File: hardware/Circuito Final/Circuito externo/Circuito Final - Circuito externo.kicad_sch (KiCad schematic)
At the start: 74 parts, among them J1 Conn_02x19_Odd_Even, J2 Conn_02x19_Odd_Even, J3 Conn_01x02, J4 Conn_01x02, J5 Conn_01x03_Pin, Q1 FDMS6681Z, Q2 FDMS6681Z, Q3 MMBT2222A, SW1 SW_SPDT, SW2 SW_DIP_x04, SW3 SW_DIP_x04, SW4 SW_DIP_x01, SW5 SW_DIP_x01, SW6 SW_DIP_x01, U1 Opamp_Quad, U2 ICL7660, U3 INA180A1

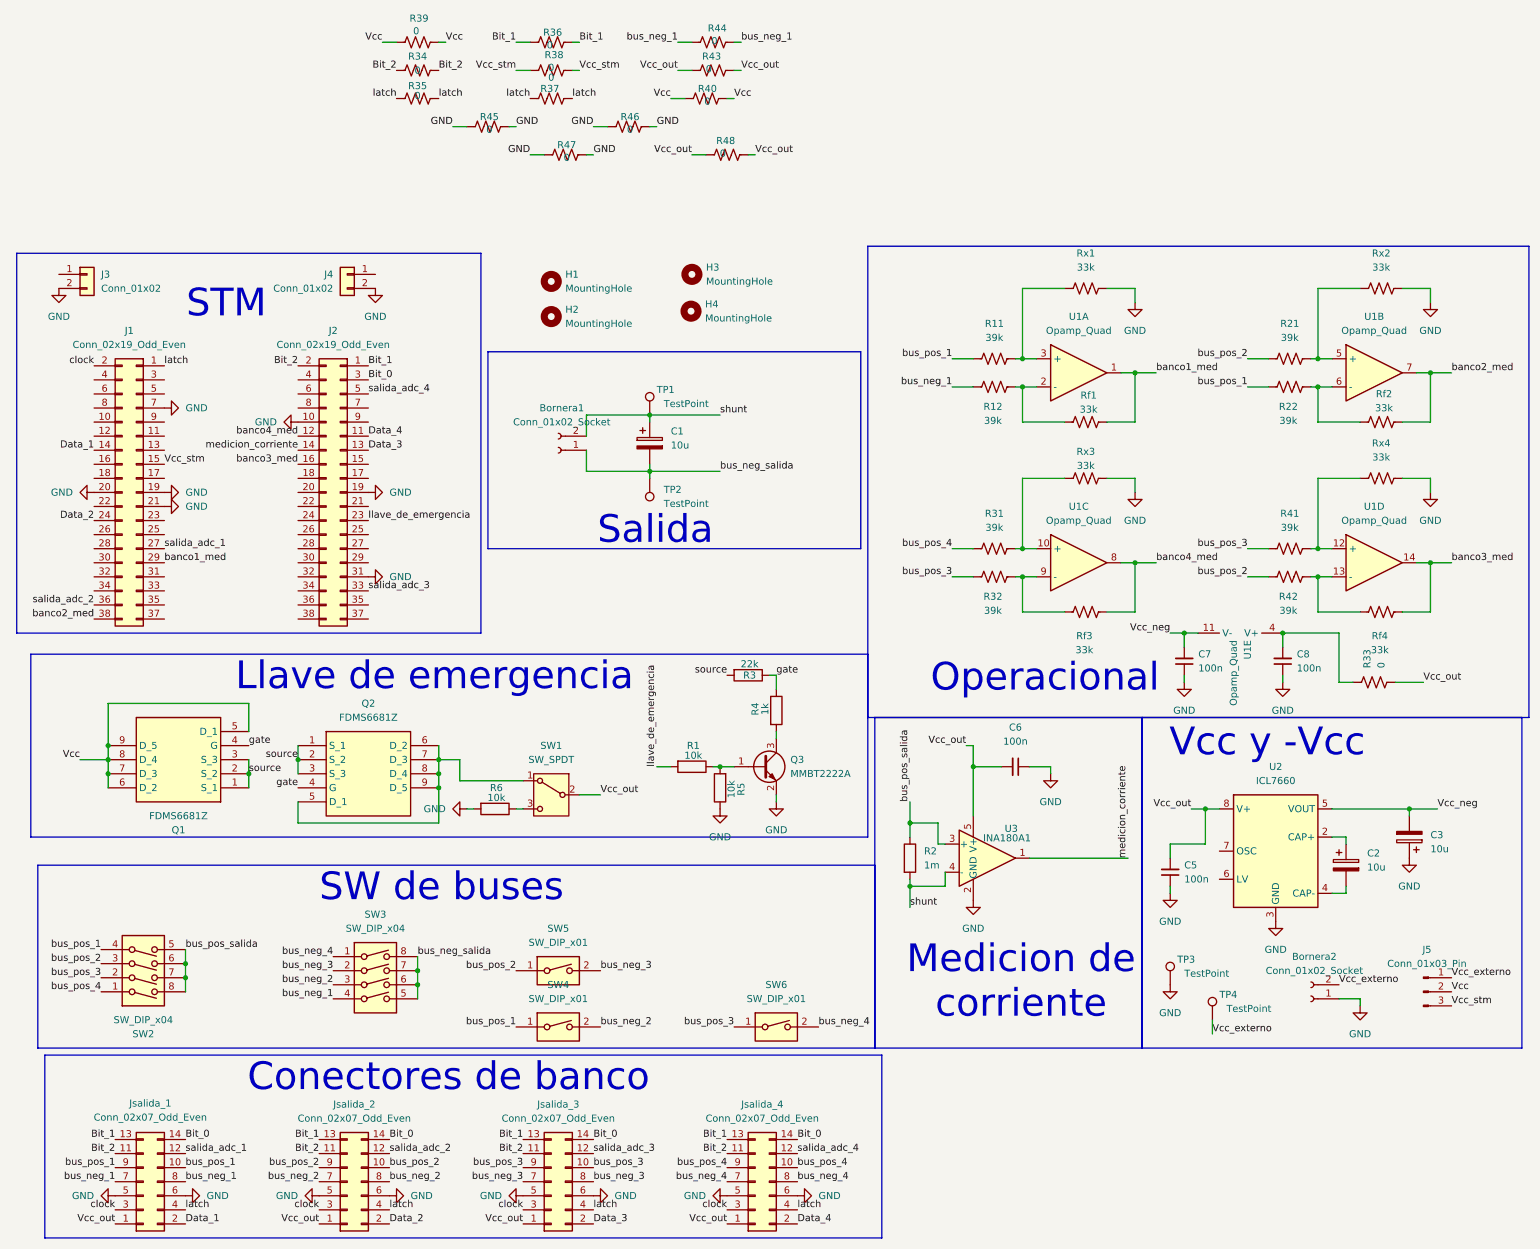
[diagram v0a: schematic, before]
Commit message: listo la placa central
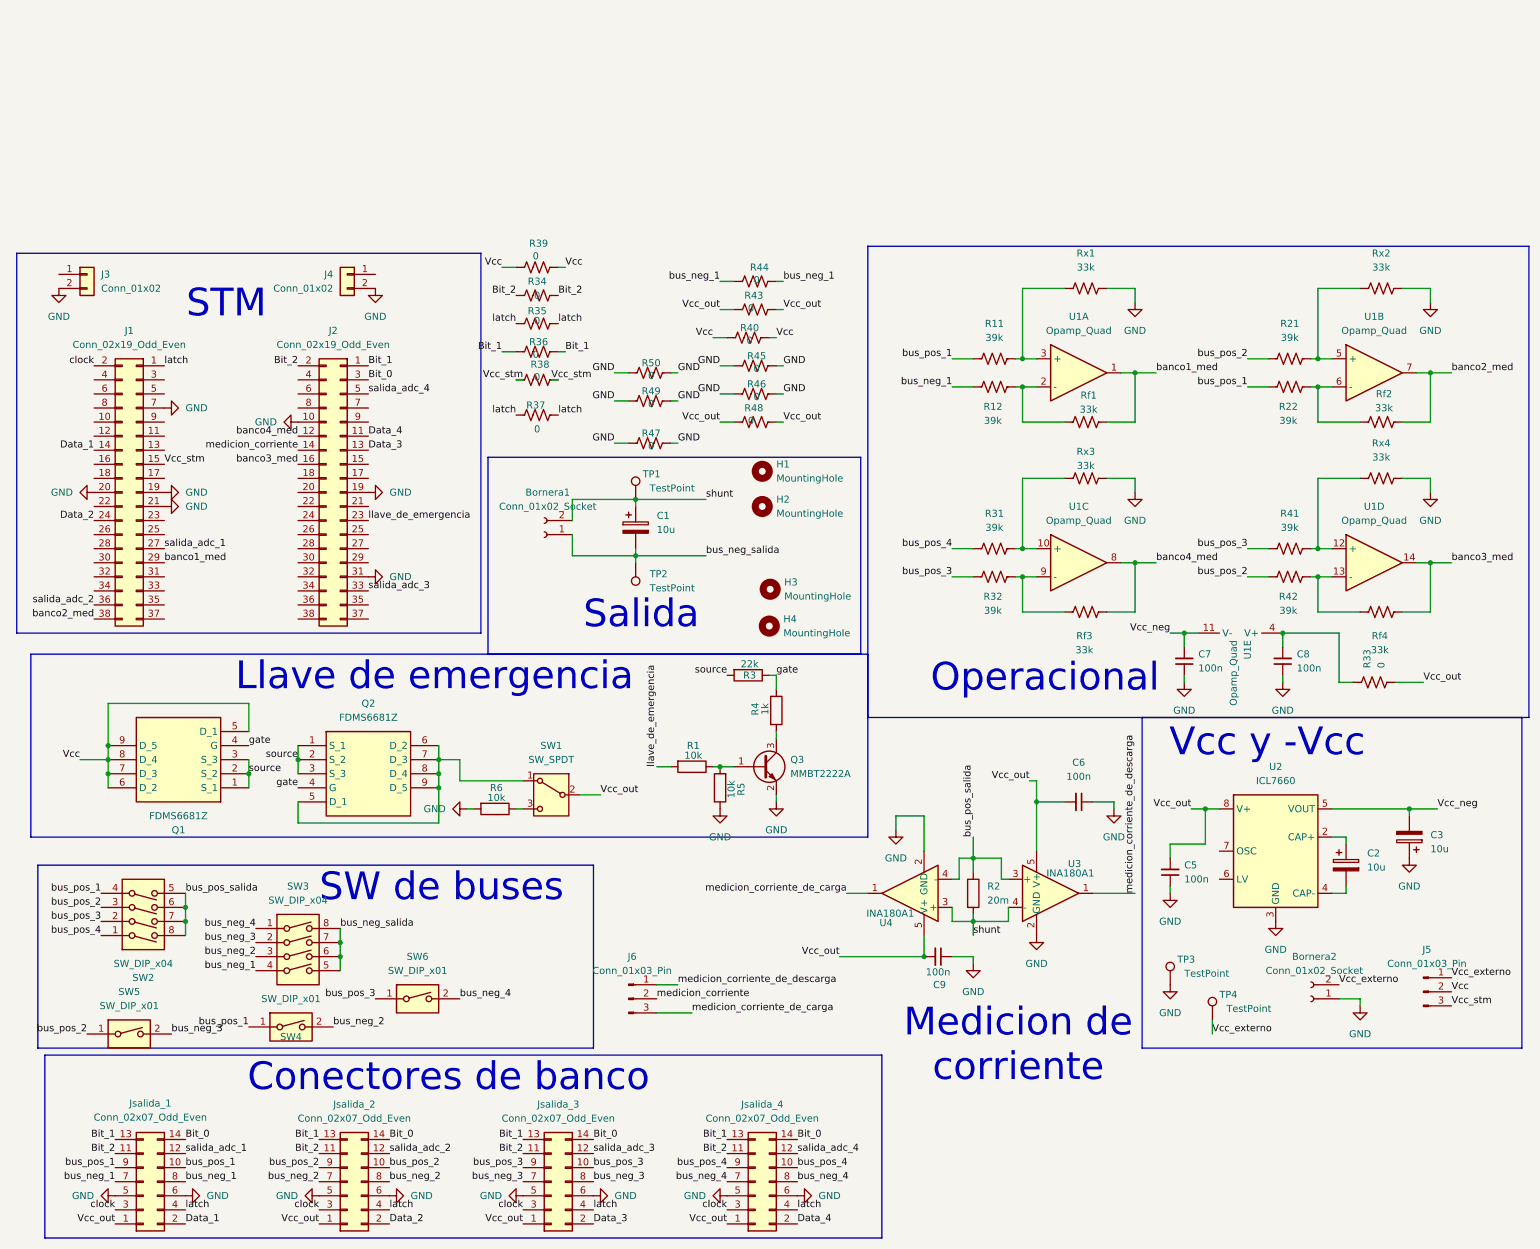
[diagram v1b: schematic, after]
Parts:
- added C9: 100n, Capacitor_SMD:C_1206_3216Metric_Pad1.33x1.80mm_HandSolder, symbol Device:C_Small
- added J6: Conn_01x03_Pin, Connector_PinHeader_2.54mm:PinHeader_1x03_P2.54mm_Vertical, symbol Connector:Conn_01x03_Pin
- added R49, R50: 0, Resistor_SMD:R_1206_3216Metric_Pad1.30x1.75mm_HandSolder, symbol Device:R_US
- added U4: INA180A1, Package_TO_SOT_SMD:SOT-23-5, symbol Amplifier_Current:INA180A1
- R2: value 1m -> 20m
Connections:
- net GND: now also C9.1, R49.1, R49.2, R50.1, R50.2, U4.2 (GND)
- net Vcc_out: now also C9.2, U4.5 (V+)
- net bus_pos_salida: now also U4.4 (-)
- net medicion_corriente: now also J6.2 (Pin_2); no longer U3.1
- net shunt: now also U4.3 (+)
- new net medicion_corriente_de_carga: J6.3 (Pin_3), U4.1
- new net medicion_corriente_de_descarga: J6.1 (Pin_1), U3.1
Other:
- moved on the sheet: Bornera1, C1, C6, H1, H2, H3, H4, R2, R34, R35, R36, R37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
